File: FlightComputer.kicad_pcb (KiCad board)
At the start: 4 copper layers, 73.7 x 73.7 mm, 88 parts, among them J1 B3B-XH-A, J3 DM3D-SF, J4 12401832E402A, U1 AP62150WU-7TSOT26-WU_DIO, U2 TPS2121RUXR, U4 RP2350_60QFN, Y1 ABM8-272-T3

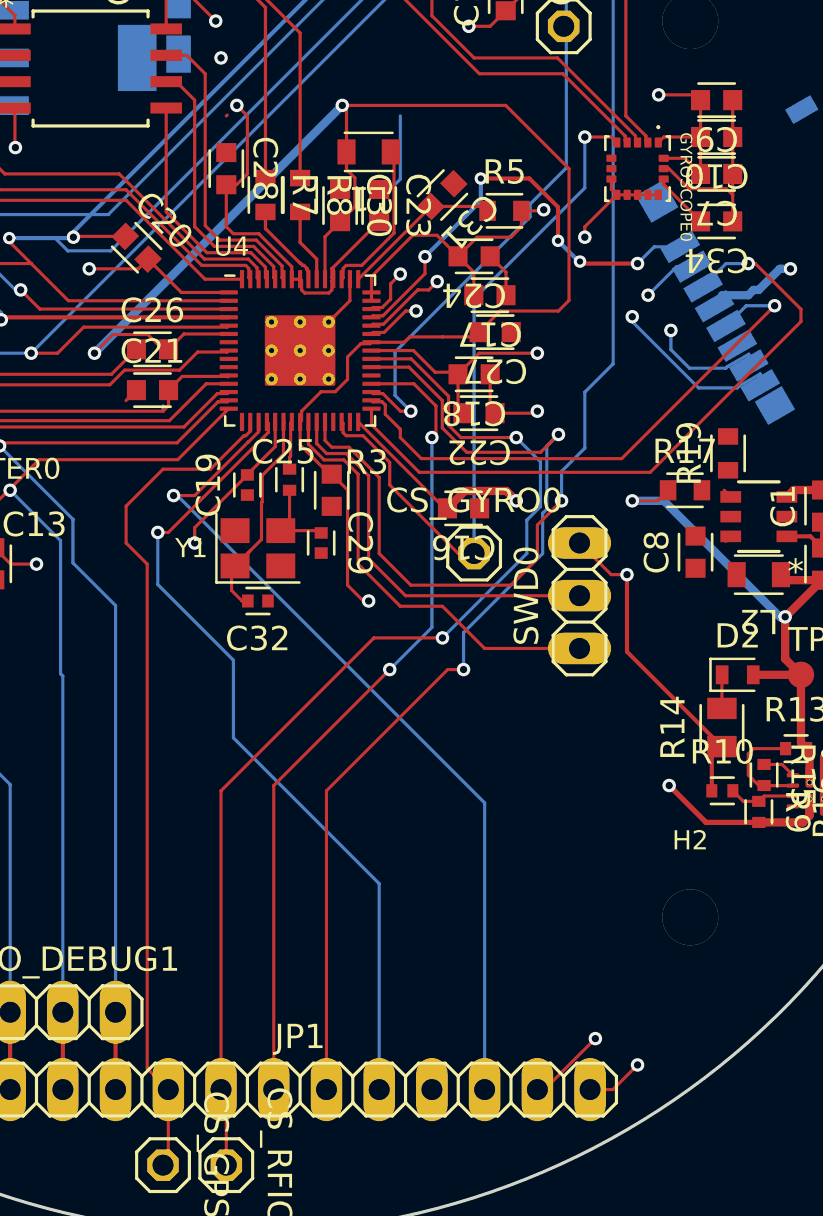
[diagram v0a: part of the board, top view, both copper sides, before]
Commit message: Meeting 1 Practice :>
Just played around with traces and components to get the hang of KiCAD!
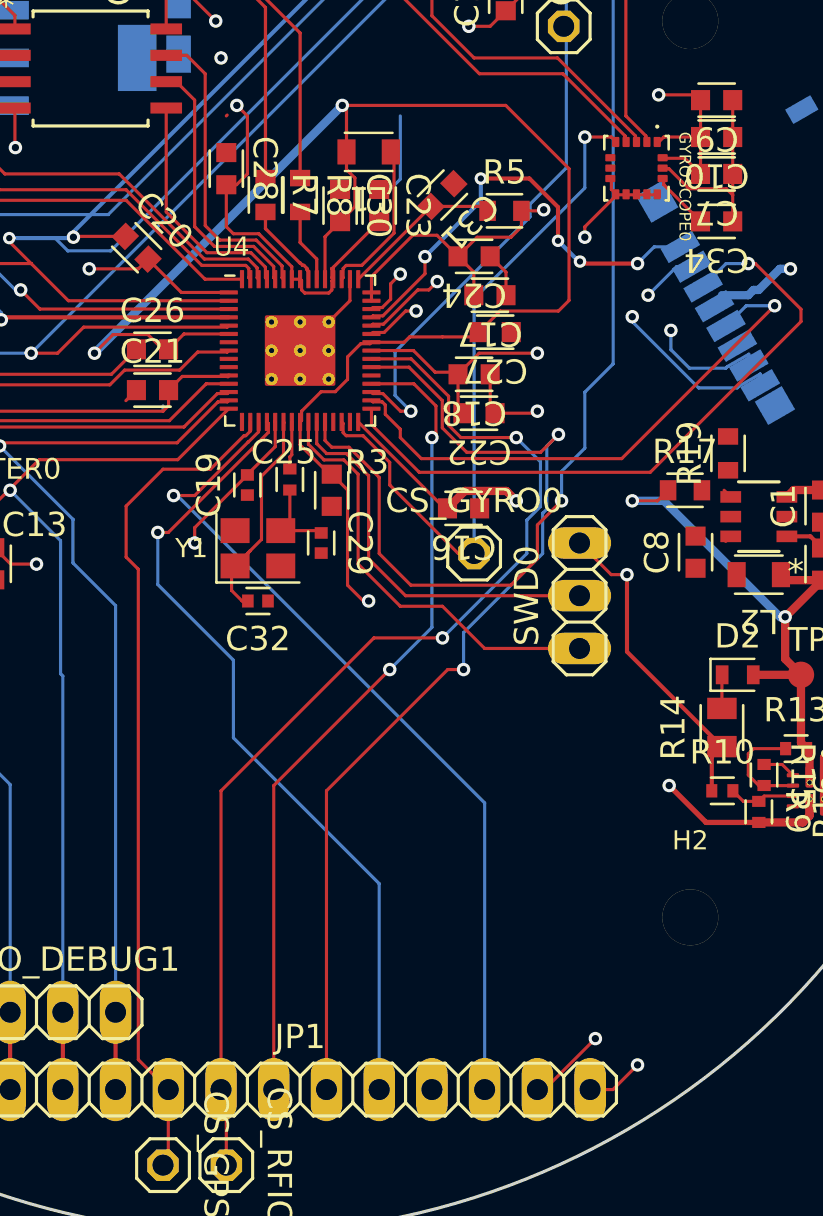
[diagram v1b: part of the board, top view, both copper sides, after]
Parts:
- moved GYROSCOPE0 0.06 mm to (167.5, 90.5)
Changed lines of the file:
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@@
 	(footprint "FlightComputer:RESC1005X40"
 		(layer "F.Cu")
-		(at 150.7871 105.5116 -90)
+		(at 150.8 105.5 -90)
 		(descr "Chip, 1.05 X 0.54 X 0.40 mm body\n\nChip package with body size 1.05 X 0.54 X 0.40 mm")
 		(property "Reference" "R3"
@@
 		)
 		(property "Datasheet" ""
-			(at 0 0 270)
+			(at 0 0 90)
 			(layer "F.Fab")
 			(hide yes)
@@
 		)
 		(property "Description" ""
-			(at 0 0 270)
+			(at 0 0 90)
 			(layer "F.Fab")
 			(hide yes)
@@
 		(pad "1" smd rect
 			(at -0.5075 0 270)
-			(size 0.5351 0.644)
+			(size 0.5355 0.644)
 			(layers "F.Cu" "F.Mask" "F.Paste")
 			(net 88 "/XOUT")
@@
 	(footprint "FlightComputer:PQFN50P300X300X80-16N"
 		(layer "F.Cu")
-		(at 167.5511 90.5256 -90)
+		(at 167.5 90.5 -90)
 		(property "Reference" "GYROSCOPE0"
 			(at -1.753268 -2.003731 270)
@@
 			(polygon
 				(pts
-					(xy 166.7511 89.7256) (xy 166.7511 91.3256) (xy 168.3511 91.3256) (xy 168.3511 89.7256)
+					(xy 166.7 89.7) (xy 166.7 91.3) (xy 168.3 91.3) (xy 168.3 89.7)
 				)
 			)
@@
 			(polygon
 				(pts
-					(xy 166.7511 89.7256) (xy 166.7511 91.3256) (xy 168.3511 91.3256) (xy 168.3511 89.7256)
+					(xy 166.7 89.7) (xy 166.7 91.3) (xy 168.3 91.3) (xy 168.3 89.7)
 				)
 			)
@@
 	)
 	(segment
-		(start 150.7871 107.5396)
-		(end 150.3631 107.9636)
+		(start 150.8 106.0075)
+		(end 150.8 107.5267)
 		(width 0.1524)
 		(layer "F.Cu")
@@
 	)
 	(segment
-		(start 150.7871 106.0191)
-		(end 150.7871 107.5396)
+		(start 152.1997 107.9636)
+		(end 152.3111 108.075)
 		(width 0.1524)
 		(layer "F.Cu")
@@
 	)
 	(segment
-		(start 152.1997 107.9636)
-		(end 152.3111 108.075)
+		(start 150.8 107.5267)
+		(end 150.3631 107.9636)
 		(width 0.1524)
 		(layer "F.Cu")
@@
 	)
 	(segment
-		(start 149.4688 105.3059)
-		(end 149.4688 106.587337)
+		(start 148.8821 108.9446)
+		(end 148.1631 109.6636)
 		(width 0.1524)
 		(layer "F.Cu")
@@
 	)
 	(segment
-		(start 149.4345 106.621637)
-		(end 149.4345 108.3882)
-		(width 0.1524)
-		(layer "F.Cu")
-		(net 24)
-	)
-	(segment
-		(start 148.8821 108.9446)
-		(end 148.1631 109.6636)
+		(start 150.4951 104.2796)
+		(end 149.4345 105.3402)
 		(width 0.1524)
 		(layer "F.Cu")
@@
 	)
 	(segment
-		(start 150.4951 104.2796)
-		(end 149.4688 105.3059)
-		(width 0.1524)
-		(layer "F.Cu")
-		(net 24)
-	)
-	(segment
 		(start 147.9931 110.0836)
 		(end 147.9931 110.8456)
@@
 	)
 	(segment
-		(start 149.4345 108.3882)
-		(end 148.8821 108.9406)
+		(start 149.4345 105.3402)
+		(end 149.4345 108.3882)
 		(width 0.1524)
 		(layer "F.Cu")
@@
 	)
 	(segment
-		(start 150.5331 102.7641)
-		(end 150.4951 102.7261)
+		(start 149.4345 108.3882)
+		(end 148.8821 108.9406)
 		(width 0.1524)
 		(layer "F.Cu")
@@
 	)
 	(segment
-		(start 149.4688 106.587337)
-		(end 149.4345 106.621637)
+		(start 150.5331 102.7641)
+		(end 150.4951 102.7261)
 		(width 0.1524)
 		(layer "F.Cu")
@@
 	)
 	(segment
-		(start 143.9291 133.874806)
-		(end 143.9291 109.5756)
-		(width 0.1524)
-		(layer "F.Cu")
-		(net 27)
-	)
-	(segment
-		(start 142.9131 106.7816)
-		(end 144.6911 105.0036)
+		(start 146.9771 105.0036)
+		(end 148.5885 103.3922)
 		(width 0.1524)
 		(layer "F.Cu")
@@
 	)
 	(segment
-		(start 144.6911 105.0036)
-		(end 146.9771 105.0036)
+		(start 142.9131 106.7816)
+		(end 144.6911 105.0036)
 		(width 0.1524)
 		(layer "F.Cu")
@@
 	)
 	(segment
-		(start 146.9771 105.0036)
-		(end 148.5885 103.3922)
+		(start 143.5 133.445706)
+		(end 143.5 109.82325)
 		(width 0.1524)
 		(layer "F.Cu")
@@
 	(segment
 		(start 144.9451 134.890806)
-		(end 143.9291 133.874806)
+		(end 143.5 133.445706)
 		(width 0.1524)
 		(layer "F.Cu")
@@
 	)
 	(segment
-		(start 144.6911 138.5316)
-		(end 144.9451 138.2776)
+		(start 144.6911 105.0036)
+		(end 146.9771 105.0036)
 		(width 0.1524)
 		(layer "F.Cu")
@@
 	)
 	(segment
-		(start 143.9291 109.5756)
-		(end 142.9131 108.5596)
+		(start 148.5885 103.3922)
+		(end 148.675143 103.3922)
 		(width 0.1524)
 		(layer "F.Cu")
@@
 	)
 	(segment
-		(start 148.675143 103.3922)
-		(end 148.8951 103.172244)
+		(start 143.5 109.82325)
+		(end 142.9131 109.23635)
 		(width 0.1524)
 		(layer "F.Cu")
@@
 	)
 	(segment
-		(start 142.9131 108.5596)
-		(end 142.9131 106.7816)
+		(start 144.6911 138.5316)
+		(end 144.9451 138.2776)
 		(width 0.1524)
 		(layer "F.Cu")
@@
 	)
 	(segment
-		(start 148.5885 103.3922)
-		(end 148.675143 103.3922)
+		(start 148.675143 103.3922)
+		(end 148.8951 103.172244)
+		(width 0.1524)
+		(layer "F.Cu")
+		(net 27)
+	)
+	(segment
+		(start 142.9131 109.23635)
+		(end 142.9131 106.7816)
 		(width 0.1524)
 		(layer "F.Cu")
@@
 	)
 	(segment
-		(start 150.7871 105.0041)
-		(end 150.7871 104.418657)
-		(width 0.1524)
-		(layer "F.Cu")
-		(net 88)
-	)
-	(segment
-		(start 150.8379 104.367857)
-		(end 150.8379 102.7833)
+		(start 150.8 104.405757)
+		(end 150.8951 104.310657)
 		(width 0.1524)
 		(layer "F.Cu")
@@
 	)
 	(segment
-		(start 150.8379 102.7833)
+		(start 150.8951 104.310657)
 		(end 150.8951 102.7261)
 		(width 0.1524)
@@
 	)
 	(segment
-		(start 150.7871 104.418657)
-		(end 150.8379 104.367857)
+		(start 150.8 104.9925)
+		(end 150.8 104.405757)
 		(width 0.1524)
 		(layer "F.Cu")
